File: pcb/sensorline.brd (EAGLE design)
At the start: 141 x 21.3 mm, 33 parts, among them X1 FH12-14S-0.5SH

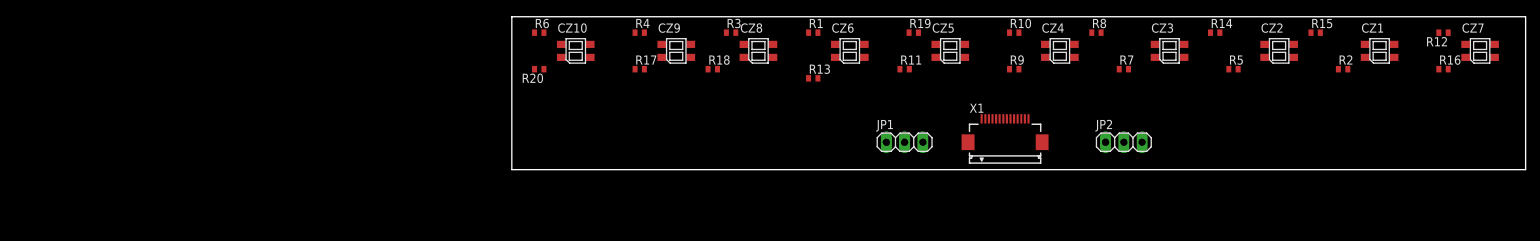
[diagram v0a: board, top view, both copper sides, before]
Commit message: o już niewiele
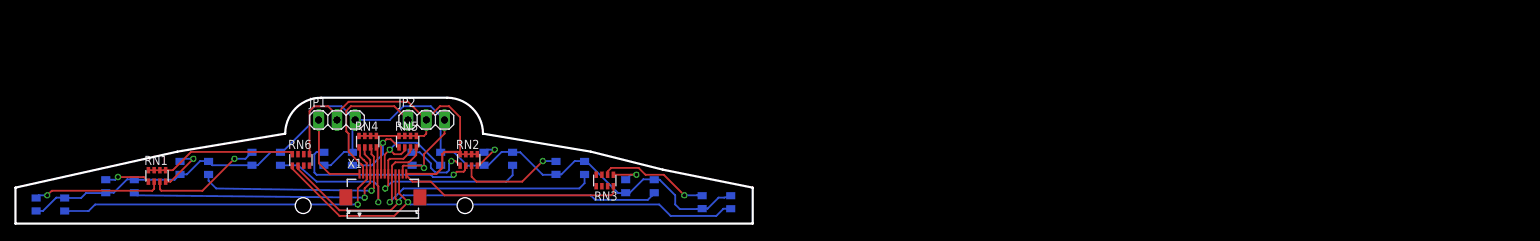
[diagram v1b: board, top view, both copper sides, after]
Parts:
- removed CZ10, CZ9: KTIR0711S, KTIR0711S:TOP
- removed R1, R10, R12, R14, R17, R19, R3, R4, R6, R8: 10k, rcl:R0402
- removed R11, R13, R15, R16, R18, R2, R20, R5, R7, R9: 330, rcl:R0402
- added CZ0, CZ19: KTIR0711S, KTIR0711S:TOP
- added RN1, RN2, RN3, RN4, RN5, RN6: CTS742C083, resistor-net:CTS742C083
- moved CZ1 176.1 mm to (-38.0, -2.30), flipped to the bottom, turned to 180 degrees
- moved CZ2 151.7 mm to (-27.6, 0.24), flipped to the bottom, turned to 180 degrees
- moved CZ7 127.5 mm to (24.6, 0.24), flipped to the bottom, turned to 180 degrees
- moved CZ3 126.5 mm to (-17.6, 1.51), flipped to the bottom, turned to 180 degrees
- moved CZ4 101.5 mm to (-7.63, 1.51), flipped to the bottom, turned to 180 degrees
- moved JP2 97.0 mm to (4.62, 6.91)
- moved X1 86.8 mm to (-1.42, -3.85)
- moved JP1 79.0 mm to (-7.81, 6.91)
- moved CZ5 74.4 mm to (4.63, 1.51), flipped to the bottom, turned to 180 degrees
- moved CZ6 51.1 mm to (14.6, 1.51), flipped to the bottom, turned to 180 degrees
- moved CZ8 25.0 mm to (34.3, -2.30), flipped to the bottom, turned to 180 degrees
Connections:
- net GND: now also CZ0.EMITER, CZ0.KATODA, CZ19.EMITER, CZ19.KATODA; no longer CZ10.EMITER, CZ10.KATODA, CZ9.EMITER, CZ9.KATODA
- net N$1: now also CZ0.ANODA, RN1.2; no longer CZ7.ANODA, R16.1
- net N$10: now also RN5.1, X1.7; no longer R8.2, X1.8
- net N$11: now also RN2.1; no longer R11.1
- net N$12: now also RN5.2, X1.8; no longer R10.2, X1.7
- net N$13: now also RN2.4; no longer R13.1
- net N$14: now also RN5.3, X1.9; no longer R12.2, X1.6
- net N$15: now also CZ7.ANODA, RN2.3; no longer CZ8.ANODA, R15.1
- net N$16: now also CZ7.KOLEKTOR, RN5.4, X1.10; no longer CZ8.KOLEKTOR, R14.2, X1.5
- net N$17: now also CZ8.ANODA, RN3.1; no longer CZ9.ANODA, R18.1
- net N$18: now also CZ8.KOLEKTOR, RN6.2, X1.11; no longer CZ9.KOLEKTOR, R17.2, X1.4
- net N$19: now also CZ19.ANODA, RN3.2; no longer CZ10.ANODA, R20.1
- net N$2: now also CZ0.KOLEKTOR, RN4.1, X1.3; no longer CZ7.KOLEKTOR, R3.2, X1.12
- net N$20: now also CZ19.KOLEKTOR, RN6.1, X1.12; no longer CZ10.KOLEKTOR, R19.2, X1.3
- net N$3: now also RN1.1; no longer R2.1
- net N$4: now also RN4.2, X1.4; no longer R1.2, X1.11
- net N$5: now also RN1.4; no longer R5.1
- net N$6: now also RN4.3, X1.5; no longer R4.2, X1.10
- net N$7: now also RN1.3; no longer R7.1
- net N$8: now also RN4.4, X1.6; no longer R6.2, X1.9
- net N$9: now also RN2.2; no longer R9.1
- net VCC: now also RN1.5, RN1.6, RN1.7, RN1.8, RN2.5, RN2.6, RN2.7, RN2.8, RN3.5, RN3.6, RN3.7, RN3.8, RN4.5, RN4.6, RN4.7, RN4.8, RN5.5, RN5.6, RN5.7, RN5.8, RN6.5, RN6.6, RN6.7, RN6.8; no longer R1.1, R10.1, R11.2, R12.1, R13.2, R14.1, R15.2, R16.2, R17.1, R18.2, R19.1, R2.2, R20.2, R3.1, R4.1, R5.2, R6.1, R7.2, R8.1, R9.2
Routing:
- net GND: track 0.00 -> 144.6 mm, vias 0 -> 1
- net VCC: track 0.00 -> 113.8 mm
- net N$20: track 0.00 -> 70.5 mm, vias 0 -> 1
- net N$18: track 0.00 -> 58.4 mm, vias 0 -> 1
- net N$2: track 0.00 -> 50.5 mm, vias 0 -> 1
- net N$4: track 0.00 -> 39.8 mm, vias 0 -> 1
- net N$16: track 0.00 -> 39.6 mm, vias 0 -> 1
- net N$6: track 0.00 -> 30.3 mm, vias 0 -> 1
- net N$14: track 0.00 -> 28.1 mm, vias 0 -> 1
- net N$9: track 0.00 -> 26.3 mm, vias 0 -> 1
- net N$8: track 0.00 -> 24.7 mm, vias 0 -> 1
- net N$22: track 0.00 -> 19.4 mm
- net N$1: track 0.00 -> 17.9 mm, vias 0 -> 1
- net N$7: track 0.00 -> 16.2 mm, vias 0 -> 1
- net N$12: track 0.00 -> 15.4 mm, vias 0 -> 1
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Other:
- board size 141 x 21.3 mm -> 102.5 x 17.5 mm

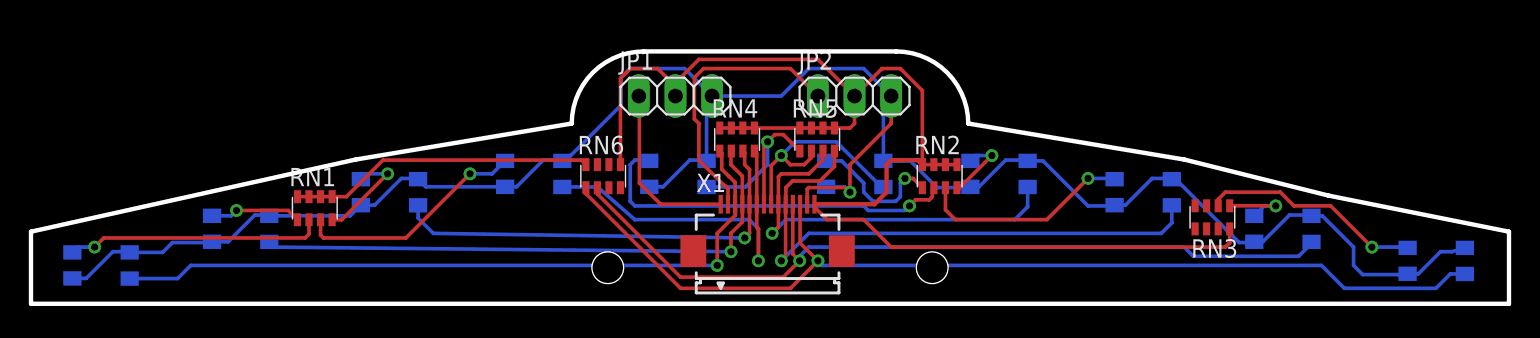
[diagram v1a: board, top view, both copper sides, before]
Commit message: hard level
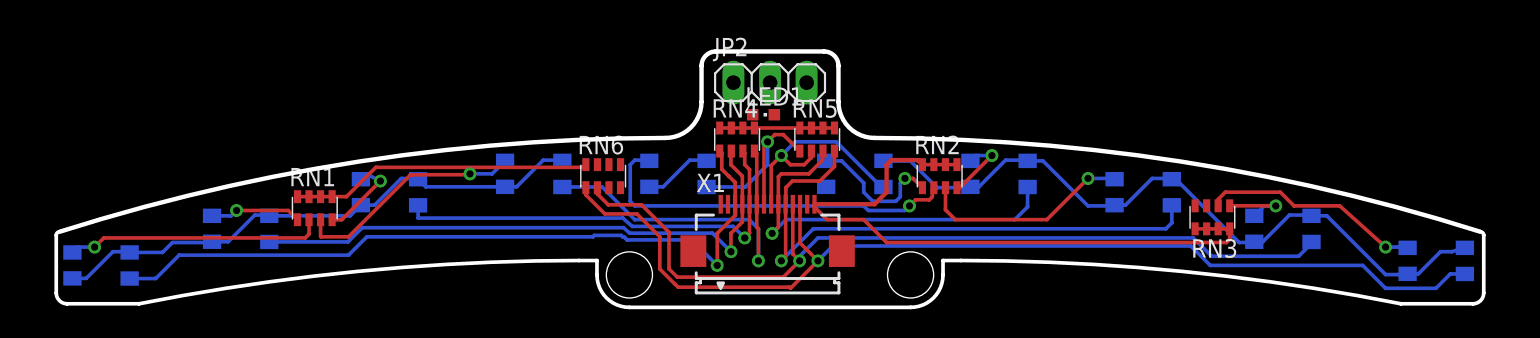
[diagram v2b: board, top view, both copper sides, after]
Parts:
- removed JP1: (no value), pinhead:1X03
- added LED1: (no value), led:CHIPLED_0603
- moved JP2 5.93 mm to (-1.25, 7.84)
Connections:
- new net N$23: LED1.C, X1.1
- net GND: no longer JP1.3
- net N$21: now also LED1.A, RN3.4; no longer JP1.1, X1.1
- net VCC: no longer JP1.2
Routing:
- net GND: track 144.6 -> 91.7 mm, vias 1 -> 0
- net VCC: track 113.8 -> 74.5 mm
- net N$22: track 19.4 -> 0.00 mm
- net N$21: track 12.3 -> 0.00 mm
- net N$20: track 70.5 -> 72.7 mm
- net N$18: track 58.4 -> 60.4 mm
- net N$2: track 50.5 -> 52.2 mm
- net N$4: track 39.8 -> 41.3 mm
- net N$5: track 7.18 -> 6.09 mm
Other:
- board size 102.5 x 17.5 mm -> 99 x 17.8 mm
